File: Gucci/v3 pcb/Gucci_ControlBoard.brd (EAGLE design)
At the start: 66 x 56 mm, 89 parts, among them U1 TEENSY_3.6_DIL, U2 ICM-20948, U3 PCA9306, U4 RFM69HCW_SMT, U5 LM393ADR, U6 AP2114H-1.8TRG1, U7 AP2114H-3.3TRG1

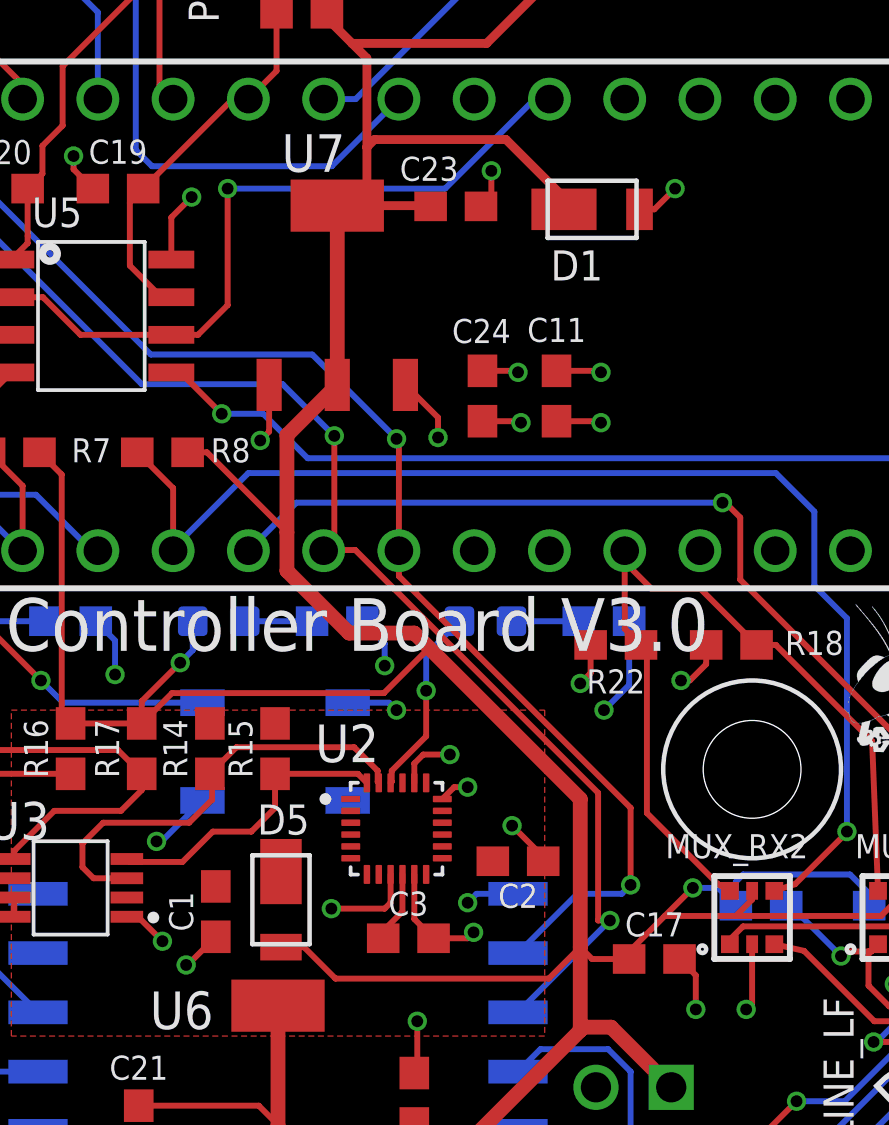
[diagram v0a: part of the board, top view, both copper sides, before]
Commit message: Replaced more parts on Gucci
Replaced more parts on Gucci
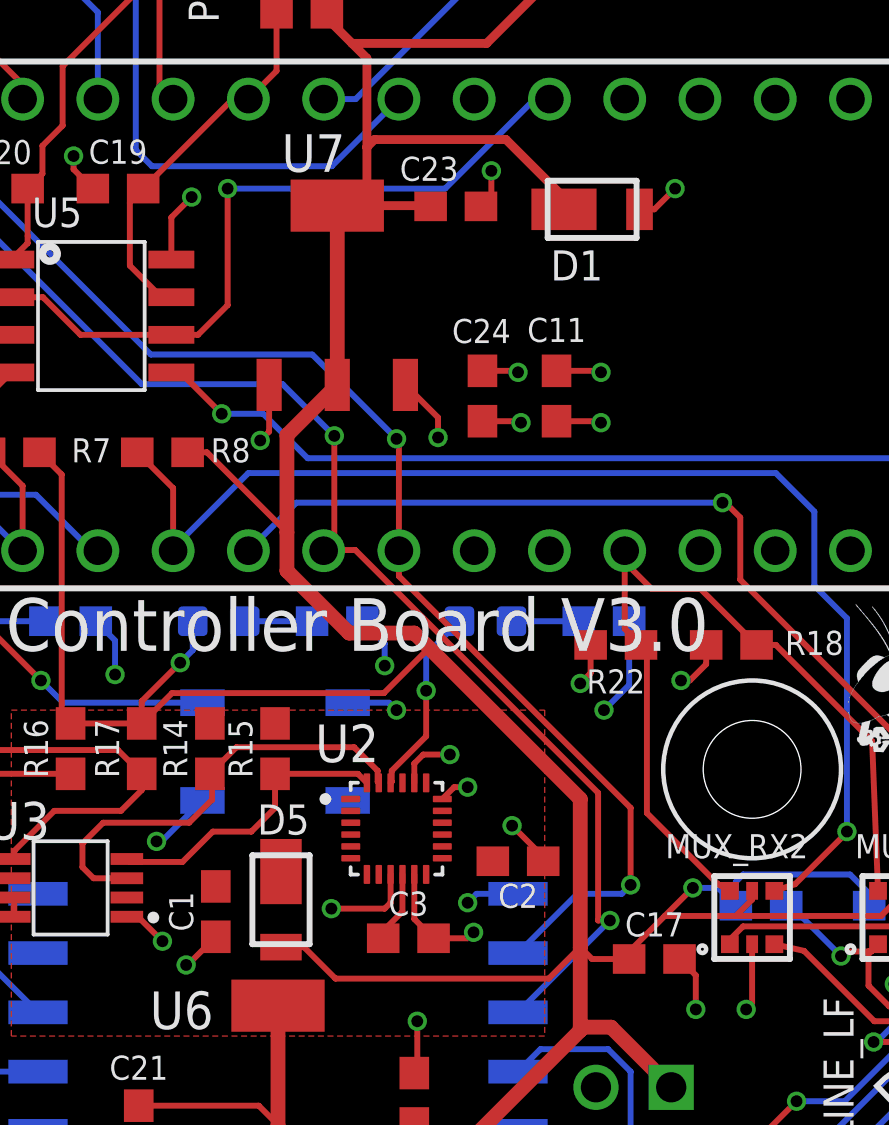
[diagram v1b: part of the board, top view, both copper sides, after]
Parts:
- D1, D5: value DFLS130L-7_30V_1A -> 30; device Kirbi_ControlBoard:DFLS130L-7_30V_1A -> Kirbi_ControlBoard:DFLS130L-7
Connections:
- net +3.3V: now also D1.2, D5.1; no longer D1.P$2, D5.P$1
- net +5V: now also D1.1; no longer D1.P$1
- net 1.8V: now also D5.2; no longer D5.P$2
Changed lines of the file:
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@@
 <attribute name="VALUE" x="30.9" y="0.838" size="0.6096" layer="28" font="vector" ratio="20" rot="MR0" align="top-center"/>
 </element>
-<element name="D1" library="Kirbi_ControlBoard" package="DFLS130L-7_30V_1A" value="DFLS130L-7_30V_1A" x="29.6" y="41.9" smashed="yes">
+<element name="D1" library="Kirbi_ControlBoard" package="DFLS130L-7" value="30" x="29.6" y="41.9" smashed="yes">
+<attribute name="DKPN" value="DFLS130LDICT-ND" x="29.6" y="41.9" size="1.778" layer="27" display="off"/>
 <attribute name="NAME" x="28.2" y="39.5" size="1.016" layer="25" font="vector"/>
-<attribute name="VALUE" x="27.6" y="39.2" size="1.016" layer="27" font="vector"/>
-</element>
-<element name="D5" library="Kirbi_ControlBoard" package="DFLS130L-7_30V_1A" value="DFLS130L-7_30V_1A" x="19.1" y="18.6" smashed="yes" rot="R270">
+<attribute name="VALUE" value="30" x="27.6" y="39.2" size="1.016" layer="27" font="vector"/>
+</element>
+<element name="D5" library="Kirbi_ControlBoard" package="DFLS130L-7" value="30" x="19.1" y="18.6" smashed="yes" rot="R270">
+<attribute name="DKPN" value="DFLS130LDICT-ND" x="19.1" y="18.6" size="1.778" layer="27" rot="R270" display="off"/>
 <attribute name="NAME" x="18.3" y="20.8" size="1.016" layer="25" font="vector"/>
-<attribute name="VALUE" x="16.4" y="20.6" size="1.016" layer="27" font="vector" rot="R270"/>
+<attribute name="VALUE" value="30" x="16.4" y="20.6" size="1.016" layer="27" font="vector" rot="R270"/>
 </element>
 <element name="R12" library="SparkFun-Resistors" library_urn="urn:adsk.eagle:library:532" package="0603" package3d_urn="urn:adsk.eagle:package:39650/1" value="1k" x="-4.4" y="22.8" smashed="yes" rot="R270">
@@
 <contactref element="C25" pad="1"/>
 <contactref element="C12" pad="1"/>
-<contactref element="D1" pad="P$1"/>
+<contactref element="D1" pad="1"/>
 <contactref element="POWER_SWITCH" pad="P"/>
 <contactref element="5V" pad="A"/>
@@
 <wire x1="6.54" y1="14" x2="8.27" y2="12.27" width="0.2" layer="16"/>
 <wire x1="8.27" y1="14.68" x2="8.27" y2="12.27" width="0.2" layer="1"/>
-<contactref element="D1" pad="P$2"/>
-<contactref element="D5" pad="P$1"/>
+<contactref element="D1" pad="2"/>
+<contactref element="D5" pad="1"/>
 <wire x1="28.65" y1="41.9" x2="28.65" y2="42.3" width="0.3" layer="1"/>
 <wire x1="28.65" y1="42.3" x2="26.6944" y2="44.2556" width="0.3" layer="1"/>
@@
 <wire x1="24" y1="25.6556" x2="24" y2="26.877" width="0.2" layer="16"/>
 <wire x1="24" y1="26.877" x2="25.123" y2="28" width="0.2" layer="16"/>
-<contactref element="D5" pad="P$2"/>
+<contactref element="D5" pad="2"/>
 </signal>
 <signal name="EXP_PAD">
